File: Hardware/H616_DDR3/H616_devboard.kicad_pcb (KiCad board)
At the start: 8 copper layers, 50 x 50 mm, 169 parts, among them J1 Micro_SD_Card_Det2, J2 HDMI_D_1.4, J3 USB_C_Receptacle_USB2.0, J4 USB_C_Receptacle_USB2.0, J5 Conn_01x40_Pin, Q1 AO3420_C358680, Q2 AO3401A, Q3 AO3401A, SW1 CK_KMS2xxG, U1 H616, U10 D3V3XA4B10LP, U11 D3V3XA4B10LP, U2 K4B8G1646D, U3 AXP305, U4 SW6206, U6 KLMBG2JETD-B041, U7 AP6256, U8 D3V3XA4B10LP, U9 D3V3XA4B10LP, Y1 24MHz

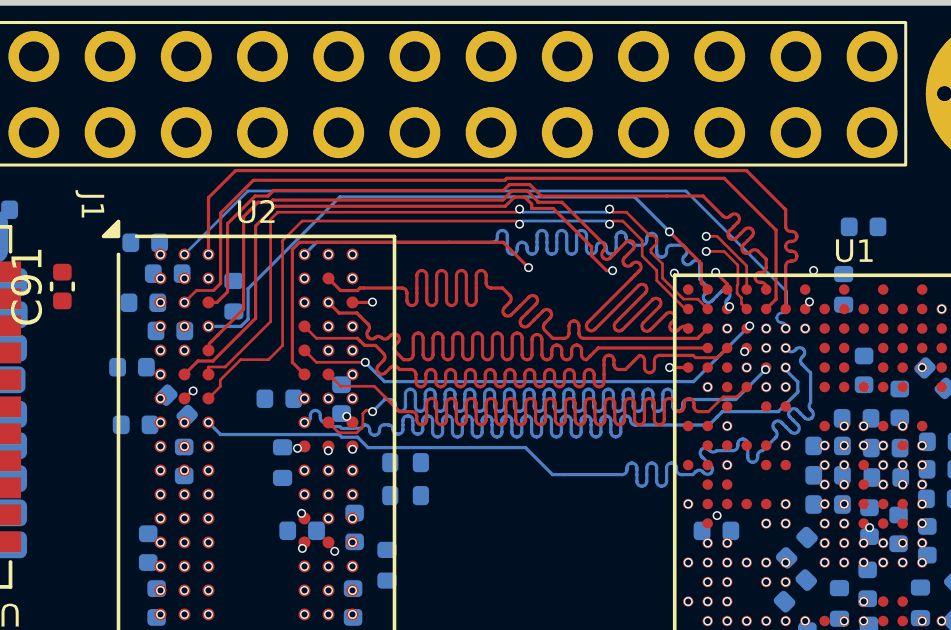
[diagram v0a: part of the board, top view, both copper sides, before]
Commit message: ddr trace. rules
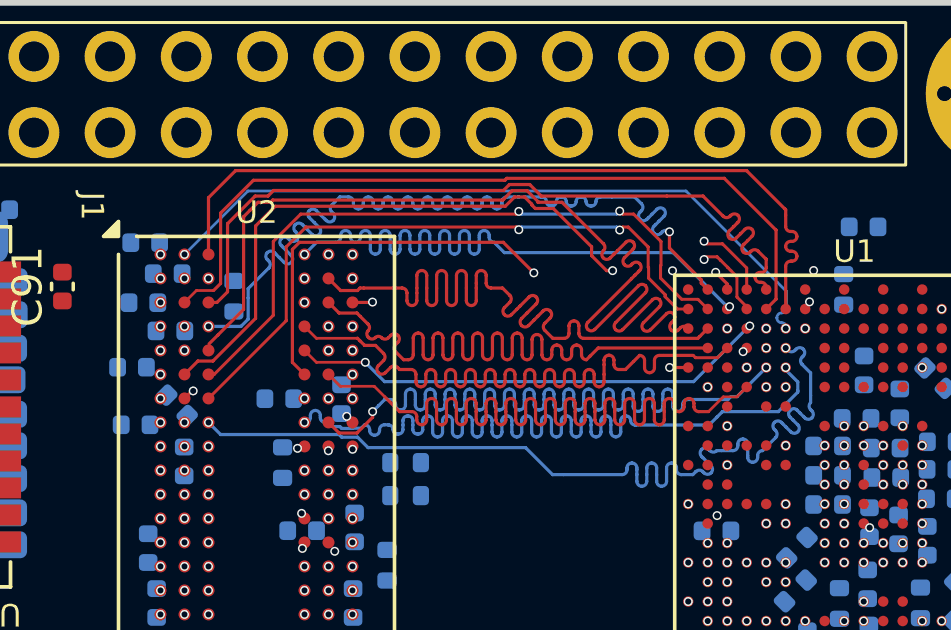
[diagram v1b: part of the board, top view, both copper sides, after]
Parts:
- R14: value 1k -> 10k
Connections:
- R14 pad 1: GND -> +3.3V
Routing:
- net /DRAM/SDQM0: track 20.7 -> 31.5 mm
- net /DRAM/DQ5: track 32.7 -> 31.5 mm
- net /DRAM/DQ12: track 24.8 -> 23.7 mm
- net /DRAM/DQ2: track 31.1 -> 30.3 mm
- net /DRAM/SDQS0P: track 17.4 -> 16.6 mm
- net /DRAM/SDQS1P: track 23.3 -> 22.5 mm
- net /DRAM/SDQS1N: track 22.5 -> 21.7 mm
- net /DRAM/DQ15: vias 1 -> 0
- net /DRAM/DQ11: vias 1 -> 0
- net /DRAM/DQ10: vias 1 -> 0

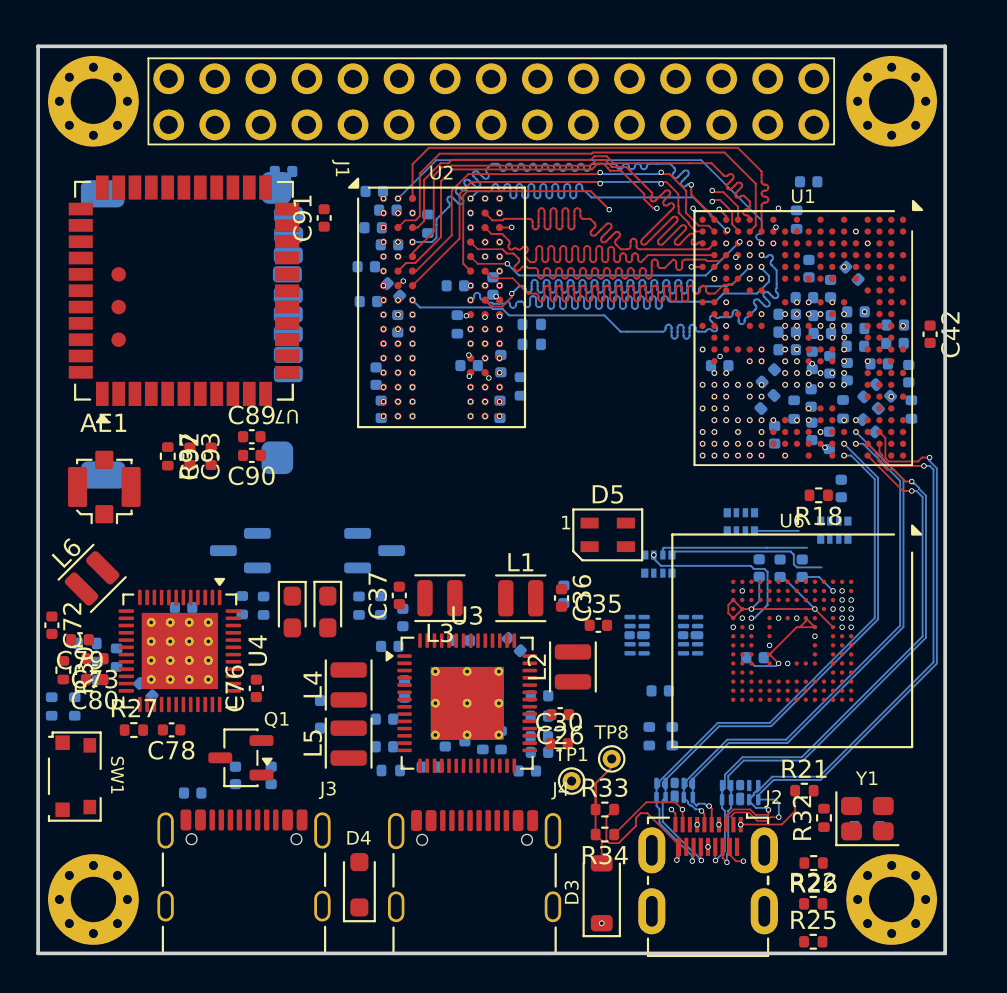
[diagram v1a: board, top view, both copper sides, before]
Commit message: ddr trace
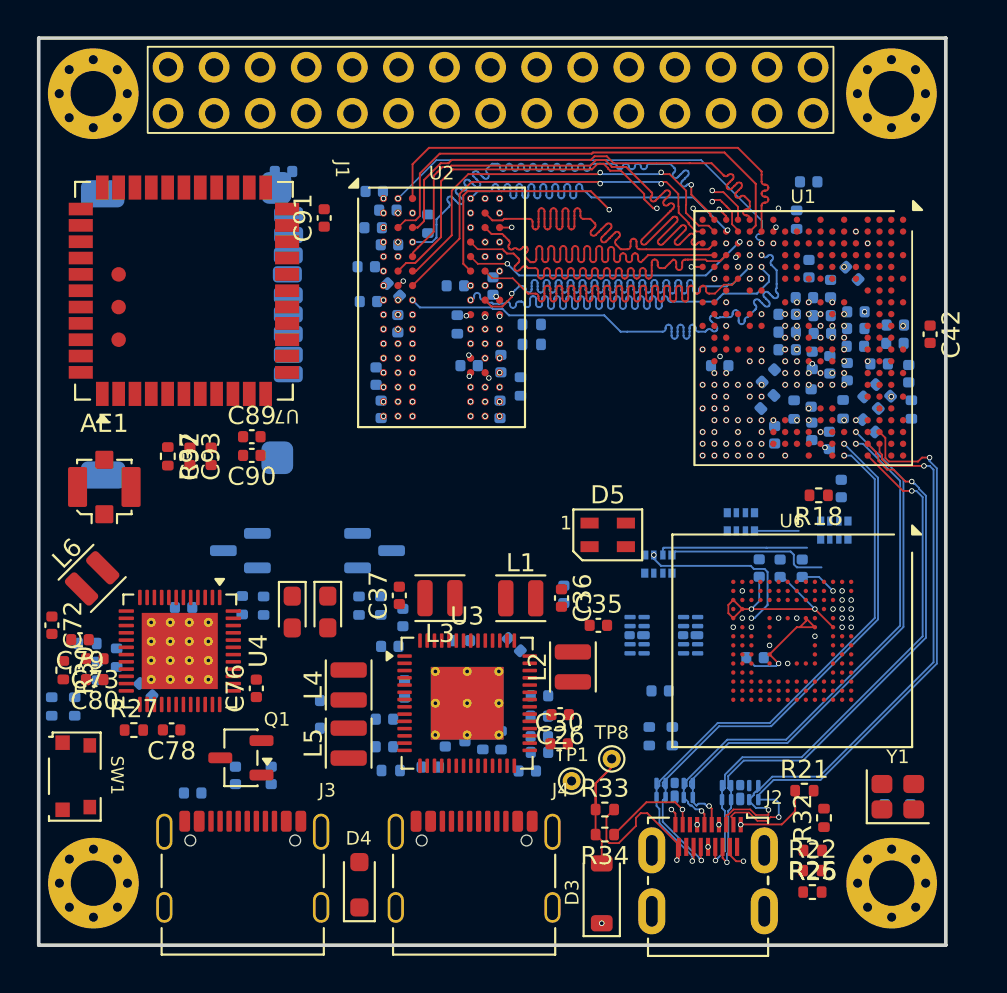
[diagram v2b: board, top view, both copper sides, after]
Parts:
- moved R25 2.74 mm to (112.7, 89.5)
- moved C59 2.07 mm to (118.1, 84.2)
- moved Y1 2.07 mm to (117.4, 84.2)
- moved C60 2.07 mm to (116.7, 84.2)
- moved R22 1.83 mm to (112.7, 88.3)
- moved H1 0.90 mm to (73.0, 89.0)
- moved H4 0.90 mm to (117.0, 89.0)
- moved R26 0.69 mm to (112.7, 87.2)
- moved J5 0.64 mm to (94.9, 45.3)
- moved H1 0.42 mm to (73.0, 45.5)
- moved H2 0.42 mm to (117.0, 45.5)
- moved J3 0.10 mm to (81.3, 88.1)
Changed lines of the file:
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@@
 			(dielectric_constraints yes)
 			(edge_connector yes)
+			(edge_plating yes)
 		)
 		(pad_to_mask_clearance 0)
@@
 	(footprint "Crystal:Crystal_SMD_2520-4Pin_2.5x2.0mm"
 		(layer "F.Cu")
-		(at 115.705 85.445)
+		(at 117.379107 84.234511)
 		(descr "SMD2520/4, Crystal, 2.5x2.0mm package, SMD, http://www.newxtal.com/UploadFiles/Images/2012-11-12-09-29-09-776.pdf")
 		(property "Reference" "Y1"
@@
 	(footprint "Resistor_SMD:R_0402_1005Metric"
 		(layer "F.Cu")
-		(at 112.74 87.89 180)
+		(at 112.691742 87.196704 180)
 		(descr "Resistor SMD 0402 (1005 Metric), square (rectangular) end terminal, IPC-7351 nominal, (Body size source: IPC-SM-782 page 72, https://www.pcb-3d.com/wordpress/wp-content/uploads/ipc-sm-782a_amendment_1_and_2.pdf)")
 		(tags "resistor")
@@
 	(footprint "MountingHole:MountingHole_2.5mm_Pad_Via"
 		(layer "F.Cu")
-		(at 73.04 89.9)
+		(at 73.04 89)
 		(descr "Mounting Hole 2.5mm, generated by kicad-footprint-generator mountinghole.py")
 		(tags "mountinghole")
@@
 	(footprint "MountingHole:MountingHole_2.5mm_Pad_Via"
 		(layer "F.Cu")
-		(at 117.04 45.9)
+		(at 117.03 45.48)
 		(descr "Mounting Hole 2.5mm, generated by kicad-footprint-generator mountinghole.py")
 		(tags "mountinghole")
@@
 	(footprint "MountingHole:MountingHole_2.5mm_Pad_Via"
 		(layer "F.Cu")
-		(at 73.04 45.9)
+		(at 73.03 45.48)
 		(descr "Mounting Hole 2.5mm, generated by kicad-footprint-generator mountinghole.py")
 		(tags "mountinghole")
@@
 	(footprint "HDR:DIP-30_100"
 		(layer "F.Cu")
-		(at 94.97 45.93)
+		(at 94.933143 45.295309)
 		(property "Reference" "J5"
 			(at -20.5 0 90)
@@
 	(footprint "Resistor_SMD:R_0402_1005Metric"
 		(layer "F.Cu")
-		(at 112.72 92.23)
+		(at 112.671383 89.490088)
 		(descr "Resistor SMD 0402 (1005 Metric), square (rectangular) end terminal, IPC-7351 nominal, (Body size source: IPC-SM-782 page 72, https://www.pcb-3d.com/wordpress/wp-content/uploads/ipc-sm-782a_amendment_1_and_2.pdf)")
 		(tags "resistor")
@@
 	(footprint "MountingHole:MountingHole_2.5mm_Pad_Via"
 		(layer "F.Cu")
-		(at 117.04 89.9)
+		(at 117.04 89)
 		(descr "Mounting Hole 2.5mm, generated by kicad-footprint-generator mountinghole.py")
 		(tags "mountinghole")
@@
 	(footprint "Connector_USB:USB_C_Receptacle_Palconn_UTC16-G"
 		(layer "F.Cu")
-		(at 81.34 88.025)
+		(at 81.27 88.095)
 		(descr "http://www.palpilot.com/wp-content/uploads/2017/05/UTC027-GKN-OR-Rev-A.pdf")
 		(tags "USB C Type-C Receptacle USB2.0")
@@
 	(footprint "Resistor_SMD:R_0402_1005Metric"
 		(layer "F.Cu")
-		(at 112.72 90.14)
+		(at 112.671742 88.306704)
 		(descr "Resistor SMD 0402 (1005 Metric), square (rectangular) end terminal, IPC-7351 nominal, (Body size source: IPC-SM-782 page 72, https://www.pcb-3d.com/wordpress/wp-content/uploads/ipc-sm-782a_amendment_1_and_2.pdf)")
 		(tags "resistor")
@@
 	(footprint "Connector_USB:USB_C_Receptacle_Palconn_UTC16-G"
 		(layer "F.Cu")
-		(at 94.05 88.06)
+		(at 94.025916 88.097347)
 		(descr "http://www.palpilot.com/wp-content/uploads/2017/05/UTC027-GKN-OR-Rev-A.pdf")
 		(tags "USB C Type-C Receptacle USB2.0")
@@
 	(footprint "Capacitor_SMD:C_0402_1005Metric"
 		(layer "B.Cu")
-		(at 114.98 85.37 90)
+		(at 116.654107 84.159511 90)
 		(descr "Capacitor SMD 0402 (1005 Metric), square (rectangular) end terminal, IPC-7351 nominal, (Body size source: IPC-SM-782 page 76, https://www.pcb-3d.com/wordpress/wp-content/uploads/ipc-sm-782a_amendment_1_and_2.pdf)")
 		(tags "capacitor")
@@
 	(footprint "Capacitor_SMD:C_0402_1005Metric"
 		(layer "B.Cu")
-		(at 116.404433 85.376856 -90)
+		(at 118.07854 84.166367 -90)
 		(descr "Capacitor SMD 0402 (1005 Metric), square (rectangular) end terminal, IPC-7351 nominal, (Body size source: IPC-SM-782 page 76, https://www.pcb-3d.com/wordpress/wp-content/uploads/ipc-sm-782a_amendment_1_and_2.pdf)")
 		(tags "capacitor")
@@
 	)
 	(gr_rect
-		(start 69.99 42.87)
-		(end 119.99 92.87)
+		(start 70.024828 42.416812)
+		(end 120.024828 92.416812)
 		(radius 2)
 		(stroke
@@
 		(last_status "tuned")
 		(last_track_width 0.1064)
-		(last_tuning_length 32.089544)
+		(last_tuning_length 32.089543)
 		(max_amplitude 0.4)
 		(min_amplitude 0.3)
@@
 		(target_delay_max 206)
 		(target_delay_min 205.8)
-		(target_length 32.089535)
+		(target_length 32.089534)
 		(target_length_max 32.103619)
 		(target_length_min 32.075451)
